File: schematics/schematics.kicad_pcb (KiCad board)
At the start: 4 copper layers, 96 x 35 mm, 35 parts, among them J1 2K, J2 SWD, J3 Micro SD Card, J4 POWER, SW1 RESET, U1 STM32F103VBT6, U2 AMS1117-3.3, Y1 16Mhz

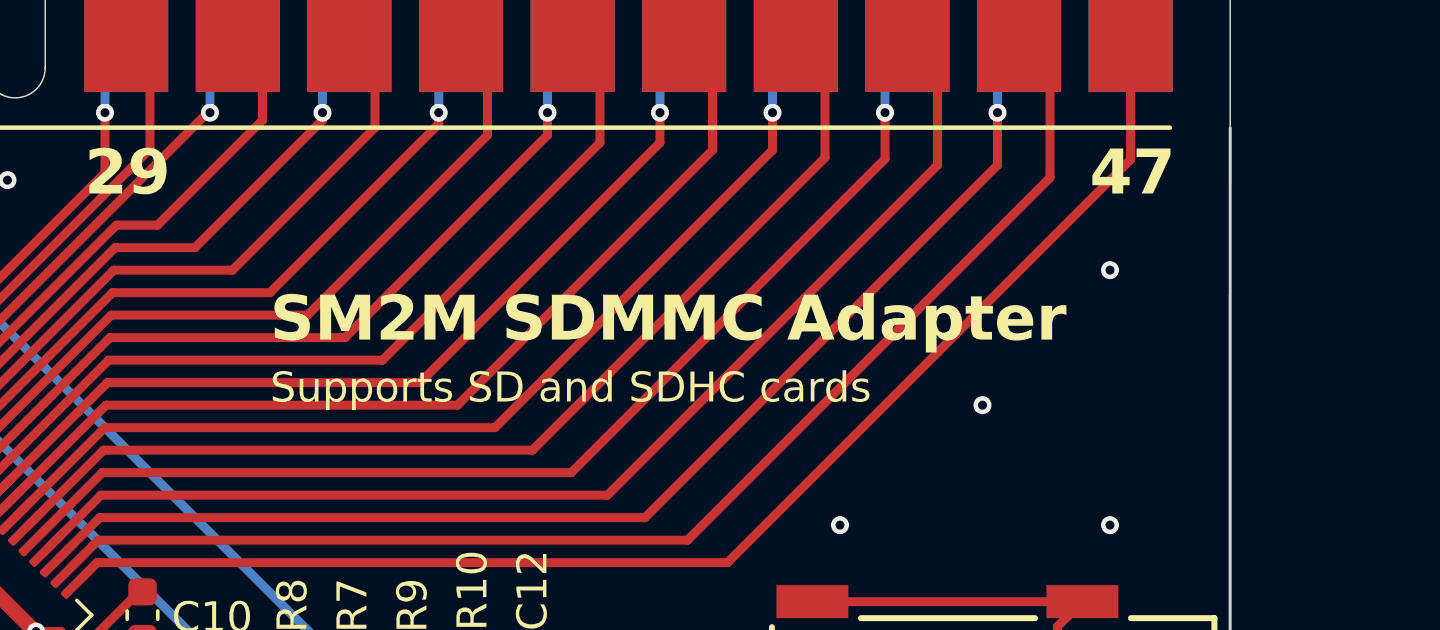
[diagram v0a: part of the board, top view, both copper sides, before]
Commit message: Update documentation
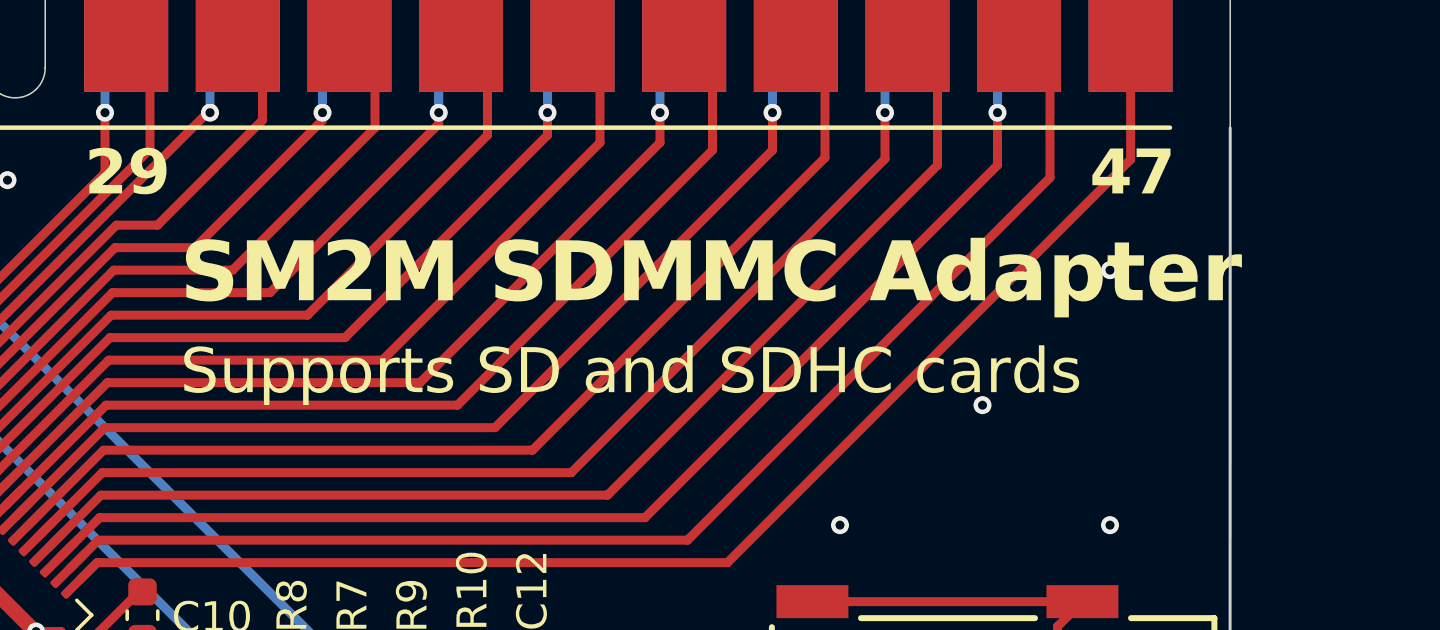
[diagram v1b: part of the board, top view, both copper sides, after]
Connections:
- net /BOOT0 renamed /MCU/BOOT0
- net /LED renamed /Power/LED
- net /VBUS renamed /Power/VBUS
- net ERR renamed ERRO
- net OSC_IN renamed Net-(U1-OSC_IN)
- net OSC_OUT renamed Net-(U1-OSC_OUT)
- net RST renamed RSTI
